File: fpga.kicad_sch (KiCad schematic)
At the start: 2 parts, among them Y1 CXO_DIP14

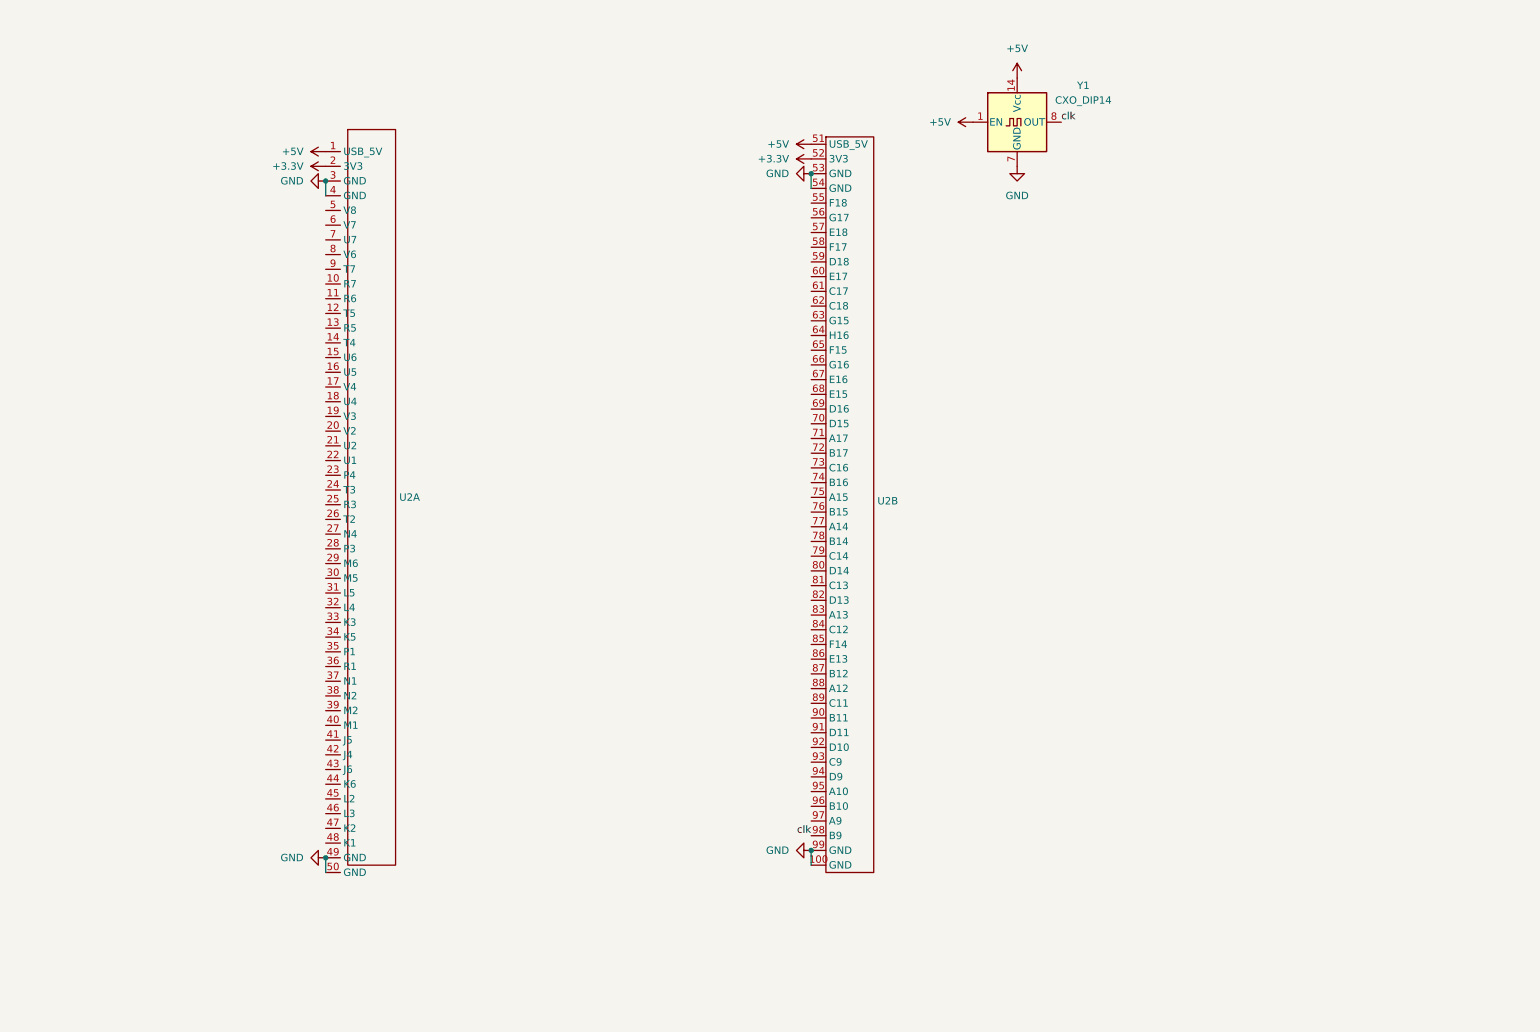
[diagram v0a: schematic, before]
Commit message: add notes
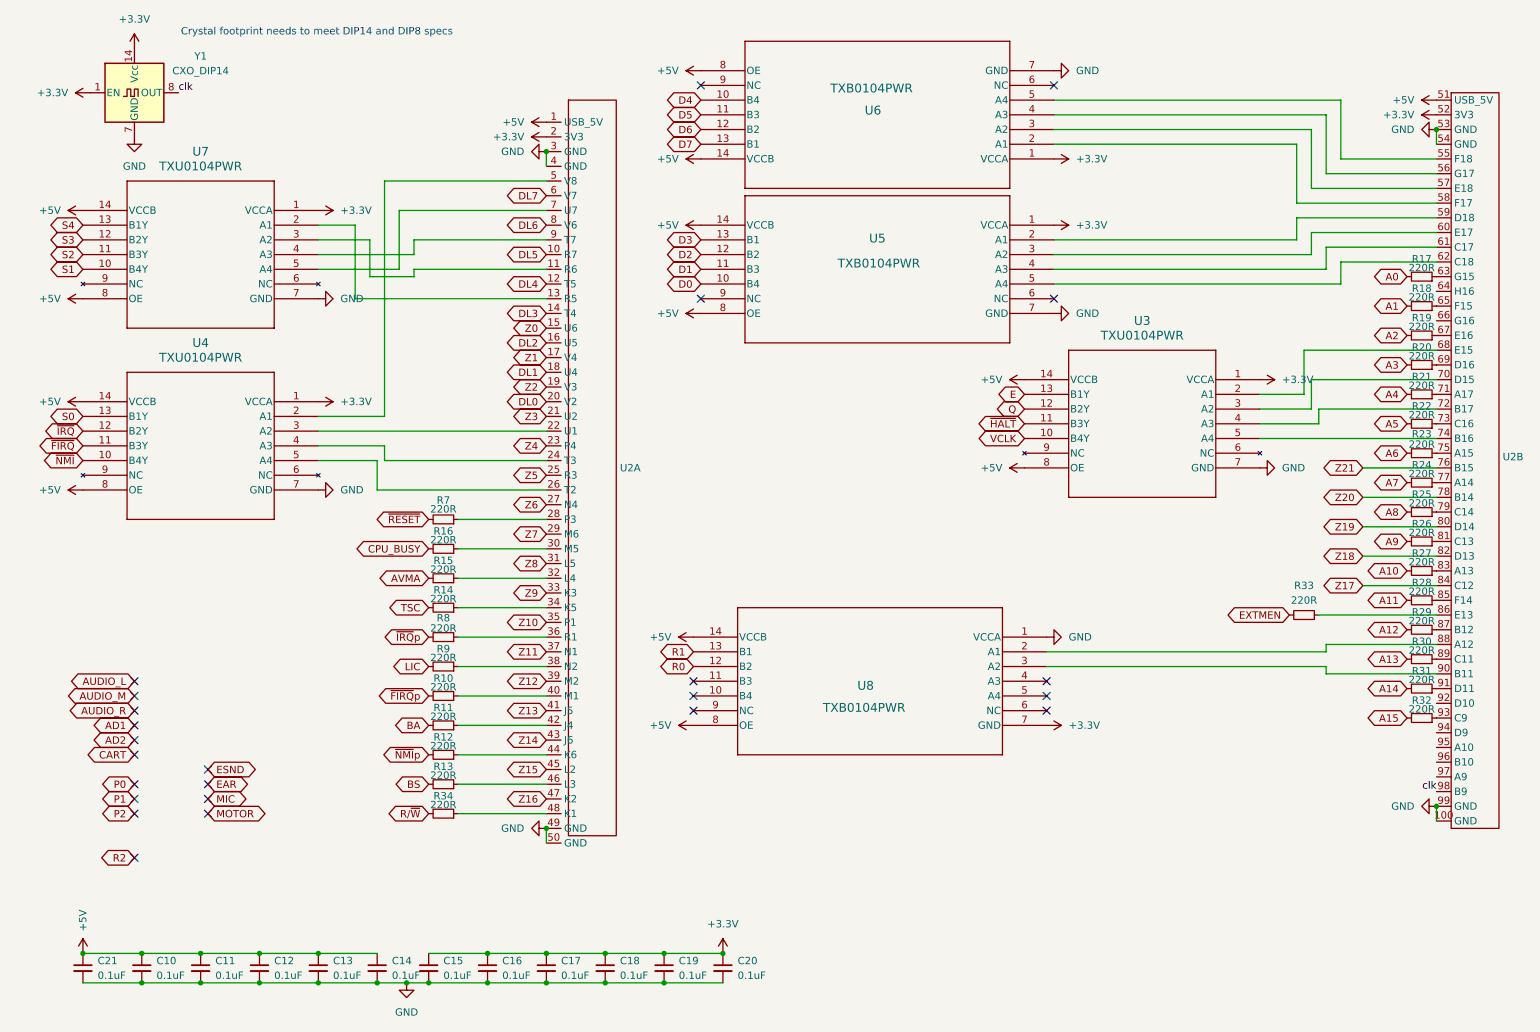
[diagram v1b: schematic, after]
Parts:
- added C10, C11, C12, C13, C14, C15, C16, C17, C18, C19, C20, C21: 0.1uF, Capacitor_SMD:C_0603_1608Metric, symbol Device:C_Small
- added R10, R11, R12, R13, R14, R15, R16, R17, R18, R19, R20, R21, R22, R23, R24, R25, R26, R27, R28, R29, R30, R31, R32, R33, R34, R7, R8, R9: 220R, Resistor_SMD:R_0603_1608Metric, symbol Device:R_Small
- added U3, U4, U7: TXU0104PWR, Library:TSSOP_0104PWR, symbol Library:TXU0104PWR
- added U5, U6, U8: TXB0104PWR, Library:TSSOP_0104PWR, symbol Library:TXB0104PWR
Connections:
- net +3.3V: now also Y1.1 (EN), Y1.14 (Vcc), C15.1, C16.1, C17.1, C18.1, C19.1, C20.1, U3.1 (VCCA), U4.1 (VCCA), U5.1 (VCCA), U6.1 (VCCA), U7.1 (VCCA), U8.7 (GND)
- net +5V: now also C10.1, C11.1, C12.1, C13.1, C14.1, C21.1, U3.14 (VCCB), U3.8 (OE), U4.14 (VCCB), U4.8 (OE), U5.14 (VCCB), U5.8 (OE), U6.14 (VCCB), U6.8 (OE), U7.14 (VCCB), U7.8 (OE), U8.14 (VCCB), U8.8 (OE); no longer Y1.1 (EN), Y1.14 (Vcc)
- net GND: now also C10.2, C11.2, C12.2, C13.2, C14.2, C15.2, C16.2, C17.2, C18.2, C19.2, C20.2, C21.2, U3.7 (GND), U4.7 (GND), U5.7 (GND), U6.7 (GND), U7.7 (GND), U8.1 (VCCA)
- net DL5: now reaches U2.10 (R7)
- net at U2.11 (R6): now also U7.3 (A2)
- net DL4: now reaches U2.12 (T5)
- net at U2.13 (R5): now also U7.2 (A1)
- net DL3: now reaches U2.14 (T4)
- net Z0: now reaches U2.15 (U6)
- net DL2: now reaches U2.16 (U5)
- net Z1: now reaches U2.17 (V4)
- net DL1: now reaches U2.18 (U4)
- net Z2: now reaches U2.19 (V3)
- net DL0: now reaches U2.20 (V2)
- net Z3: now reaches U2.21 (U2)
- net at U2.22 (U1): now also U4.3 (A2)
- net Z4: now reaches U2.23 (P4)
- net at U2.24 (T3): now also U4.4 (A3)
- net Z5: now reaches U2.25 (R3)
- net at U2.26 (T2): now also U4.5 (A4)
- net Z6: now reaches U2.27 (N4)
- net at U2.28 (P3): now also R7.1
- net Z7: now reaches U2.29 (M6)
- net at U2.30 (M5): now also R16.1
- net Z8: now reaches U2.31 (L5)
- net at U2.32 (L4): now also R15.1
- net Z9: now reaches U2.33 (K3)
- net at U2.34 (K5): now also R14.1
- net Z10: now reaches U2.35 (P1)
- net at U2.36 (R1): now also R8.1
- net Z11: now reaches U2.37 (N1)
- net at U2.38 (N2): now also R9.1
- net Z12: now reaches U2.39 (M2)
- net at U2.40 (M1): now also R10.1
- net Z13: now reaches U2.41 (J5)
- net at U2.42 (J4): now also R11.1
- net Z14: now reaches U2.43 (J6)
- net at U2.44 (K6): now also R12.1
- net Z15: now reaches U2.45 (L2)
- net at U2.46 (L3): now also R13.1
- net Z16: now reaches U2.47 (K2)
- net at U2.48 (K1): now also R34.1
- net at U2.5 (V8): now also U4.2 (A1)
- net DL7: now reaches U2.6 (V7)
- net at U2.7 (U7): now also U7.5 (A4)
- net DL6: now reaches U2.8 (V6)
- net at U2.9 (T7): now also U7.4 (A3)
- net at U2.55 (F18): now also U6.5 (A4)
- net at U2.56 (G17): now also U6.4 (A3)
- net at U2.57 (E18): now also U6.3 (A2)
- net at U2.58 (F17): now also U6.2 (A1)
- net at U2.59 (D18): now also U5.2 (A1)
- net at U2.60 (E17): now also U5.3 (A2)
- net at U2.61 (C17): now also U5.4 (A3)
- net at U2.62 (C18): now also U5.5 (A4)
- net at U2.63 (G15): now also R17.1
- net at U2.65 (F15): now also R18.1
- net at U2.67 (E16): now also R19.1
- net at U2.68 (E15): now also U3.2 (A1)
- net at U2.69 (D16): now also R20.1
- net at U2.70 (D15): now also U3.3 (A2)
- net at U2.71 (A17): now also R21.1
- net at U2.72 (B17): now also U3.4 (A3)
- net at U2.73 (C16): now also R22.1
- net at U2.74 (B16): now also U3.5 (A4)
- net at U2.75 (A15): now also R23.1
- net Z21: now reaches U2.76 (B15)
- net at U2.77 (A14): now also R24.1
- net Z20: now reaches U2.78 (B14)
- net at U2.79 (C14): now also R25.1
- net Z19: now reaches U2.80 (D14)
- net at U2.81 (C13): now also R26.1
- net Z18: now reaches U2.82 (D13)
- net at U2.83 (A13): now also R27.1
- net Z17: now reaches U2.84 (C12)
- net at U2.85 (F14): now also R28.1
- net at U2.86 (E13): now also R33.1
- net at U2.87 (B12): now also R29.1
- net at U2.88 (A12): now also U8.2 (A1)
- net at U2.89 (C11): now also R30.1
- net at U2.90 (B11): now also U8.3 (A2)
- net at U2.91 (D11): now also R31.1
- net at U2.93 (C9): now also R32.1
- new net A0: R17.2
- new net A1: R18.2
- new net A10: R27.2
- new net A11: R28.2
- new net A12: R29.2
- new net A13: R30.2
- new net A14: R31.2
- new net A15: R32.2
- new net A2: R19.2
- new net A3: R20.2
- new net A4: R21.2
- new net A5: R22.2
- new net A6: R23.2
- new net A7: R24.2
- new net A8: R25.2
- new net A9: R26.2
- new net AVMA: R15.2
- new net BA: R11.2
- new net BS: R13.2
- new net CPU_BUSY: R16.2
- new net D0: U5.10 (B4)
- new net D1: U5.11 (B3)
- new net D2: U5.12 (B2)
- new net D3: U5.13 (B1)
- new net D4: U6.10 (B4)
- new net D5: U6.11 (B3)
- new net D6: U6.12 (B2)
- new net D7: U6.13 (B1)
- new net E: U3.13 (B1Y)
- new net EXTMEN: R33.2
- new net LIC: R9.2
- new net Q: U3.12 (B2Y)
- new net R0: U8.12 (B2)
- new net R1: U8.13 (B1)
- new net R/~{W}: R34.2
- new net S0: U4.13 (B1Y)
- new net S1: U7.10 (B4Y)
- new net S2: U7.11 (B3Y)
- new net S3: U7.12 (B2Y)
- new net S4: U7.13 (B1Y)
- new net TSC: R14.2
- new net VCLK: U3.10 (B4Y)
- new net ~{FIRQ}: U4.11 (B3Y)
- new net ~{FIRQ}p: R10.2
- new net ~{HALT}: U3.11 (B3Y)
- new net ~{IRQ}: U4.12 (B2Y)
- new net ~{IRQ}p: R8.2
- new net ~{NMI}: U4.10 (B4Y)
- new net ~{NMI}p: R12.2
- new net ~{RESET}: R7.2
- no-connect marks 0 -> 24
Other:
- note added: "Crystal footprint needs to meet DIP14 and DIP8 specs"
- moved on the sheet: U2A, U2B, Y1
